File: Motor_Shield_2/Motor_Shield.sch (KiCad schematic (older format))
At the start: 42 parts, among them J1 Conn_01x08_Female, J10 Conn_01x02_Male, J11 Conn_01x02_Male, J12 Conn_01x02_Male, J13 Conn_01x02_Male, J14 Conn_01x02_Male, J15 Conn_01x02_Male, J16 Conn_01x02_Male, J17 Conn_01x02_Male, J18 Conn_01x02_Male, J19 Conn_01x02_Male, J2 Conn_01x06_Female, J20 Conn_01x02_Male, J21 Conn_01x02_Male, J22 Conn_01x02_Male, J23 Conn_01x04_Female, J3 Conn_01x08_Female, J4 Conn_01x10_Female, J5 Conn_01x02_Female, J6 Screw_Terminal_01x06, J7 Conn_01x02_Male, J8 Conn_01x02_Male, J9 Conn_01x02_Male, U1 L6474PD

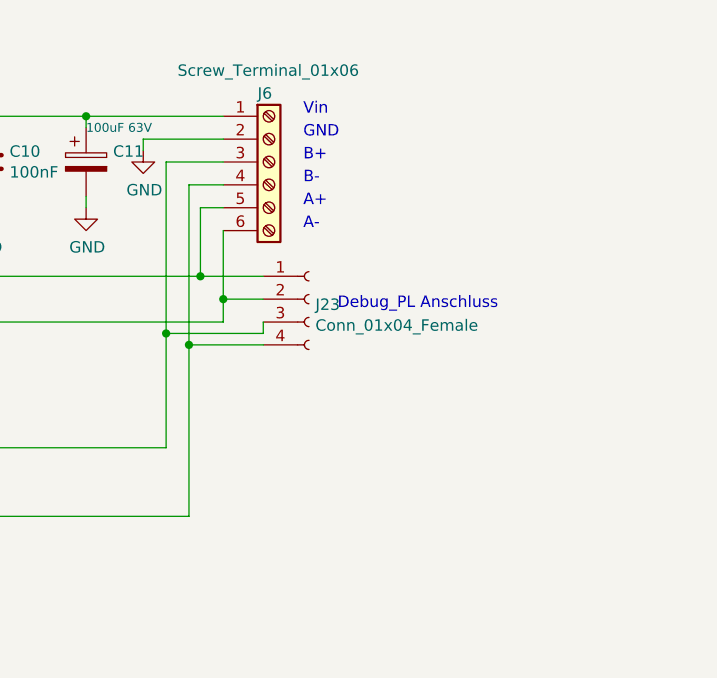
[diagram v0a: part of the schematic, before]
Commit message: PCB fertig
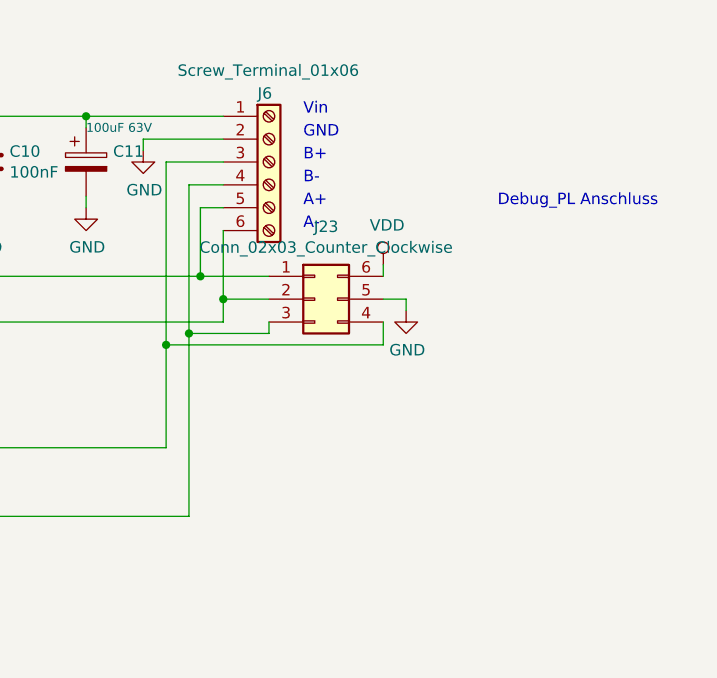
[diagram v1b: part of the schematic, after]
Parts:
- removed J23: Conn_01x04_Female, Connector_PinHeader_2.54mm:PinHeader_1x04_P2.54mm_Vertical, symbol Connector:Conn_01x04_Female
- added J23: Conn_02x03_Counter_Clockwise, Connector_PinHeader_2.54mm:PinHeader_2x03_P2.54mm_Vertical, symbol Connector_Generic:Conn_02x03_Counter_Clockwise
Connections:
- net GND: now also J23.5 (Pin_5)
- net VDD: now also J23.6 (Pin_6)
- net at J6.3 (Pin_3), U1.17 (OUT1B), U1.18 (OUT1B): now also J23.4 (Pin_4)
- net at J6.5 (Pin_5), U1.2 (OUT1A), U1.3 (OUT1A): now also J23.1 (Pin_1)
- net at J6.4 (Pin_4), U1.20 (OUT2B), U1.21 (OUT2B): now also J23.3 (Pin_3)
- net at J6.6 (Pin_6), U1.35 (OUT2A), U1.36 (OUT2A): now also J23.2 (Pin_2)
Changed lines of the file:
@@
 EESchema Schematic File Version 4
-LIBS:Motor_Shield-cache
 EELAYER 30 0
 EELAYER END
@@
 	8050 2700 8150 2700
 Connection ~ 6800 3000
-Wire Wire Line
-	8150 3200 8150 3100
 Connection ~ 6800 3200
-Wire Wire Line
-	7900 3750 7900 3250
 Wire Wire Line
 	7900 2500 8150 2500
@@
 Wire Wire Line
 	6800 3000 8050 3000
-$Comp
-L Connector:Conn_01x04_Female J23
-U 1 1 5E62AB36
-P 8525 3100
-F 0 "J23" H 8553 3076 50  0000 L CNN
-F 1 "Conn_01x04_Female" H 8553 2985 50  0000 L CNN
-F 2 "Connector_PinHeader_2.54mm:PinHeader_1x04_P2.54mm_Vertical" H 8525 3100 50  0001 C CNN
-F 3 "~" H 8525 3100 50  0001 C CNN
-	1    8525 3100
-	1    0    0    -1
-$EndComp
-Wire Wire Line
-	8050 3000 8325 3000
-Connection ~ 8050 3000
-Wire Wire Line
-	8150 3100 8325 3100
-Connection ~ 8150 3100
-Wire Wire Line
-	8150 3100 8150 2800
-Wire Wire Line
-	8325 3300 8000 3300
-Wire Wire Line
-	8000 2600 8000 3300
-Connection ~ 8000 3300
-Wire Wire Line
-	8000 3300 8000 4050
-Wire Wire Line
-	7900 3250 8325 3250
-Wire Wire Line
-	8325 3250 8325 3200
-Connection ~ 7900 3250
-Wire Wire Line
-	7900 3250 7900 2500
-Text Notes 8650 3150 0    50   ~ 0
+Text Notes 9350 2700 0    50   ~ 0
 Debug_PL Anschluss
 Text Notes 9950 5500 0    50   ~ 0
@@
 Text Notes 9275 5500 0    50   ~ 0
 J9\n\nJ14\n\nJ19\n\nJ22\n
+Wire Wire Line
+	8000 2600 8000 3250
+Wire Wire Line
+	7900 2500 7900 3300
+Wire Wire Line
+	8150 2800 8150 3100
+Wire Wire Line
+	8350 3000 8050 3000
+Connection ~ 8050 3000
+Wire Wire Line
+	8350 3100 8150 3100
+Connection ~ 8150 3100
+Wire Wire Line
+	8150 3100 8150 3200
+Wire Wire Line
+	8000 3250 8350 3250
+Wire Wire Line
+	8350 3250 8350 3200
+Connection ~ 8000 3250
+Wire Wire Line
+	8000 3250 8000 4050
+Connection ~ 7900 3300
+Wire Wire Line
+	7900 3300 7900 3750
+$Comp
+L power:VDD #PWR019
+U 1 1 5E6617F8
+P 8850 2950
+F 0 "#PWR019" H 8850 2800 50  0001 C CNN
+F 1 "VDD" H 8867 3123 50  0000 C CNN
+F 2 "" H 8850 2950 50  0001 C CNN
+F 3 "" H 8850 2950 50  0001 C CNN
+	1    8850 2950
+	1    0    0    -1
+$EndComp
+$Comp
+L power:GND #PWR021
+U 1 1 5E662C51
+P 8950 3150
+F 0 "#PWR021" H 8950 2900 50  0001 C CNN
+F 1 "GND" H 8955 2977 50  0000 C CNN
+F 2 "" H 8950 3150 50  0001 C CNN
+F 3 "" H 8950 3150 50  0001 C CNN
+	1    8950 3150
+	1    0    0    -1
+$EndComp
+$Comp
+L Connector_Generic:Conn_02x03_Counter_Clockwise J23
+U 1 1 5E69254C
+P 8550 3100
+F 0 "J23" H 8600 3417 50  0000 C CNN
+F 1 "Conn_02x03_Counter_Clockwise" H 8600 3326 50  0000 C CNN
+F 2 "Connector_PinHeader_2.54mm:PinHeader_2x03_P2.54mm_Vertical" H 8550 3100 50  0001 C CNN
+F 3 "~" H 8550 3100 50  0001 C CNN
+	1    8550 3100
+	1    0    0    -1
+$EndComp
+Wire Wire Line
+	8850 3300 8850 3200
+Wire Wire Line
+	7900 3300 8850 3300
+Wire Wire Line
+	8850 2950 8850 3000
+Wire Wire Line
+	8850 3100 8950 3100
+Wire Wire Line
+	8950 3100 8950 3150
 $EndSCHEMATC
